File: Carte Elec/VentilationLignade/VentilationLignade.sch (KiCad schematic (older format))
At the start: 48 parts, among them P1 RelaisBoard1, P10 SDCard, P11 Codeur Rotatif, P12 Teensy Bottom, P13 EndStops1, P14 Teensy_Haut, P15 EndStops2, P16 Teensy_cote, P17 Retour 12V, P18 Masse_12V, P19 12V1, P2 PUIT_CAN, P20 12V2, P21 12V_1et2, P22 Teensy_Bas, P23 Serial, P24 CHEMINEE, P25 RT_CLK1, P26 RT_CLK2, P3 RelaisBoard2, P4 TEMP_EXT, P5 RelaisBoard3, P6 TEMP_INT, P7 RelaisBoard4, P8 RelaisBoard5, P9 TFT, SW2 BackLight_On/ff

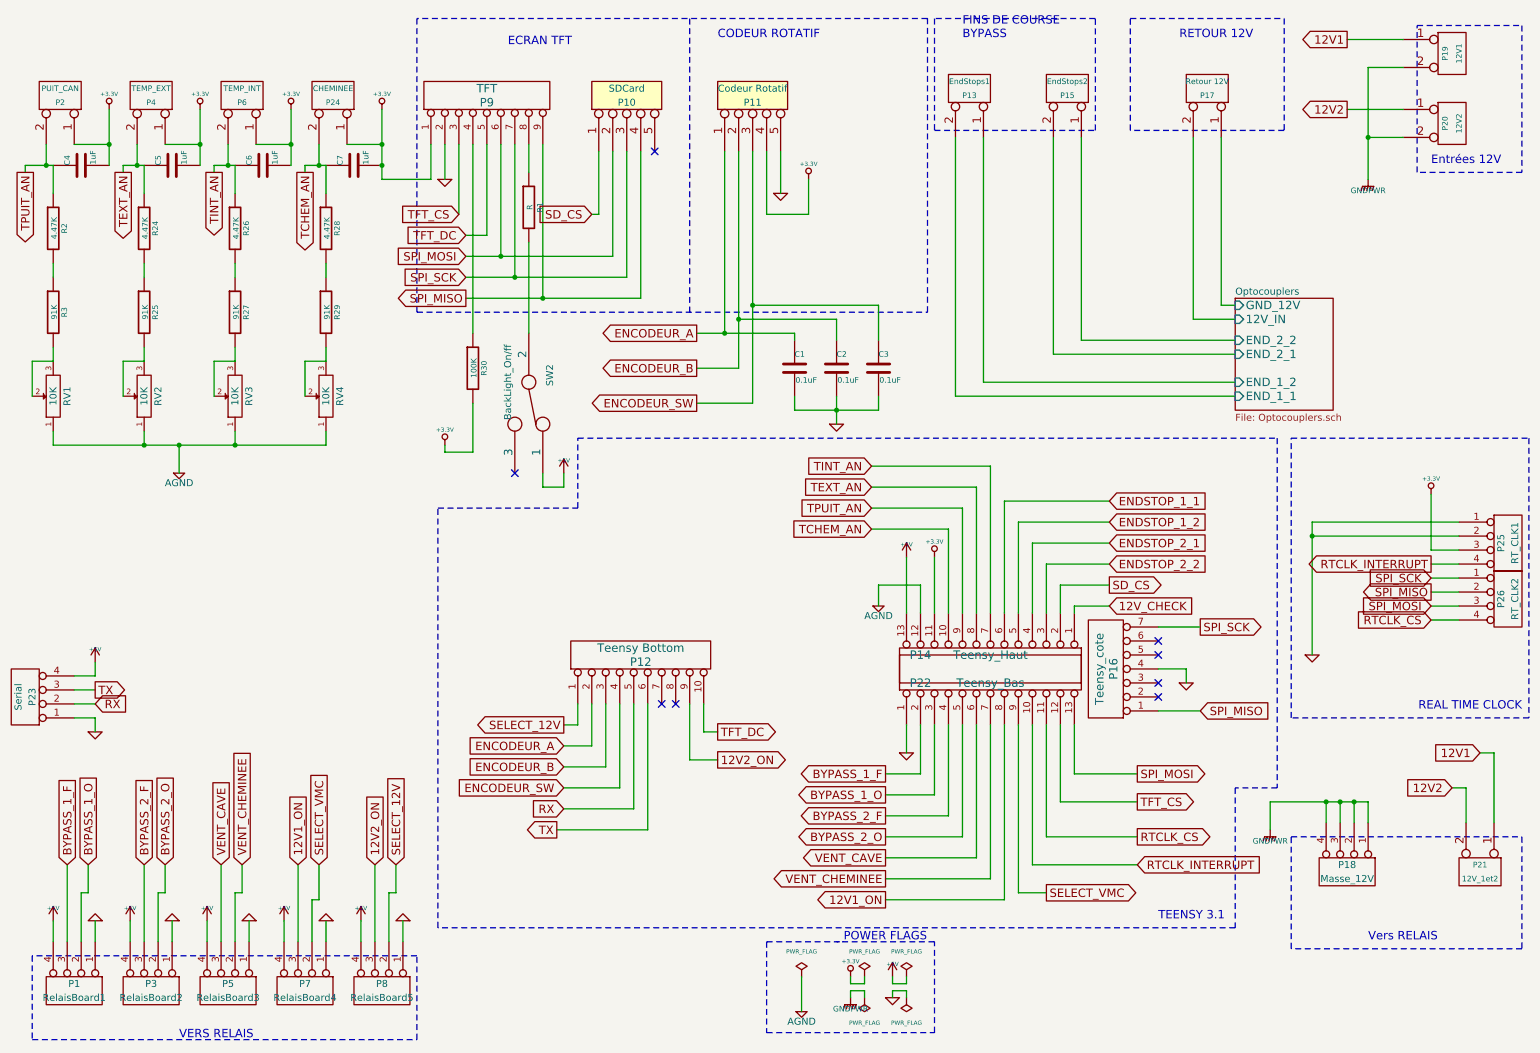
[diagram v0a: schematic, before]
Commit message: Carte a reprendre
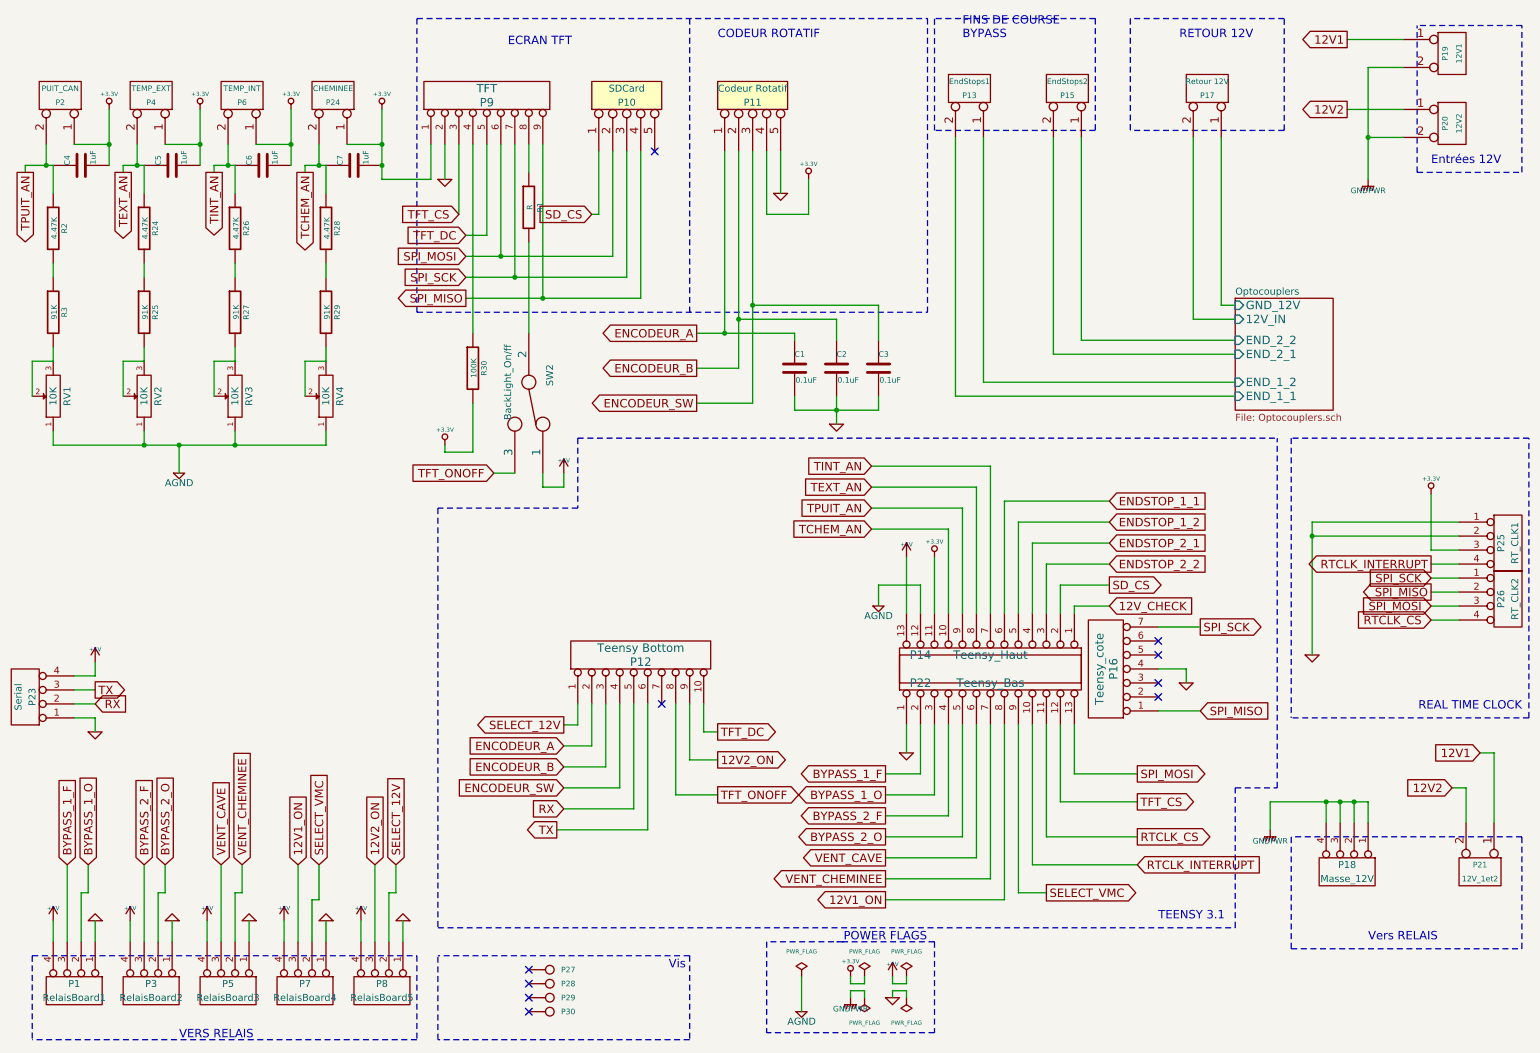
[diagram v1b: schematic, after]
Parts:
- added P27, P28, P29, P30: CONN_1, symbol CONN_1
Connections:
- net TFT_ONOFF: now reaches SW2.3
- net TFT_ONOFF: now also P12.8 (P8)
- no-connect marks 8 -> 10
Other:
- note added: "Vis"

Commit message: Modif de la carte => Commande SEEED !!!
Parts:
- removed P19: 12V1, Connect:bornier2, symbol CONN_2
- removed P20: 12V2, Connect:bornier2, symbol CONN_2
- added P19, P20: CONN_01X03, emp:Alim, symbol CONN_01X03
- P27, P28, P29, P30: footprint (none) -> emp:VIS
- RV1, RV2, RV3, RV4: footprint Potentiometers:Potentiometer_Bourns_3339S_Angular_ScrewFront -> emp:Potar; symbol POT -> POT-RESCUE-VentilationLignade
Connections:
- net 12V1: now also P19.1 (P1)
- net 12V2: now also P20.1 (P1)
- net GNDPWR: now also P19.2 (P2), P19.3 (P3), P20.2 (P2), P20.3 (P3)
